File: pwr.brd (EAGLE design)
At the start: 79.5 x 58 mm, 44 parts, among them Q1 IPD65R600C6, T1 750811647, U1 UCC28700, U3 ESP-WROOM-32

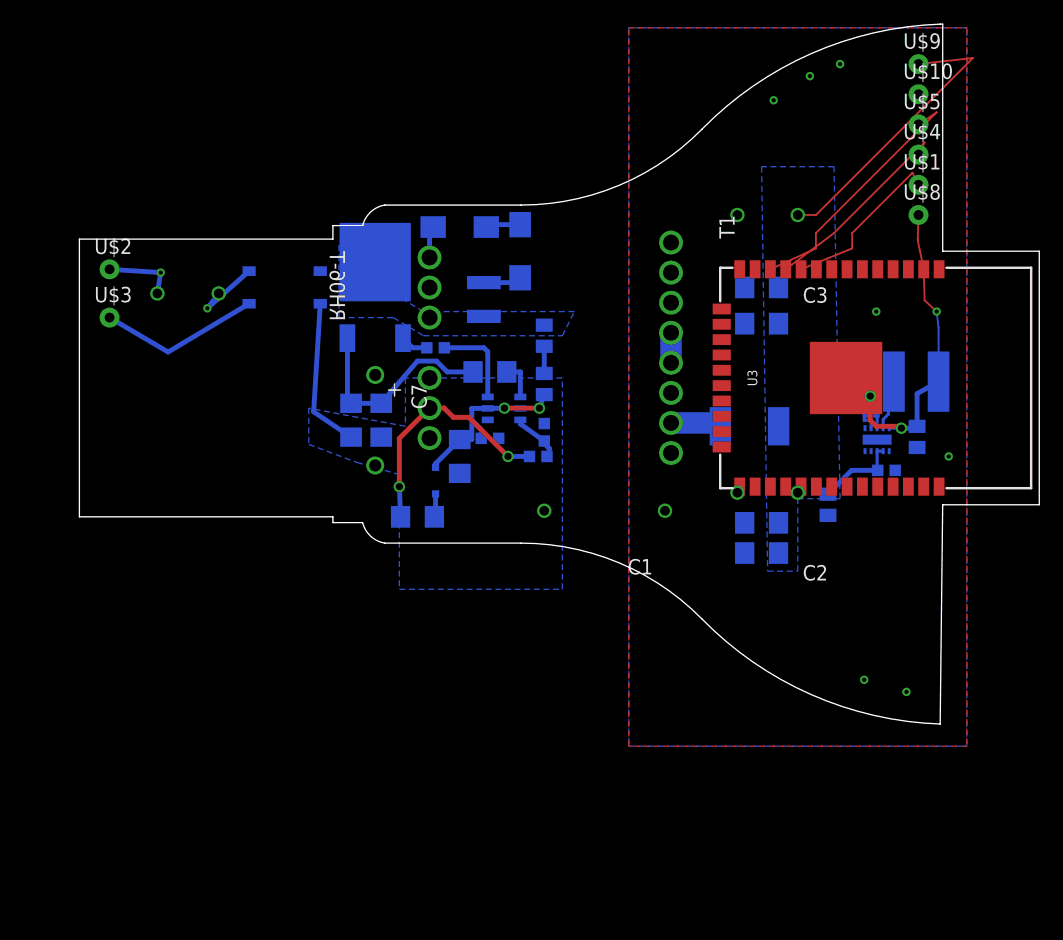
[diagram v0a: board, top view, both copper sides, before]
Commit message: ordered
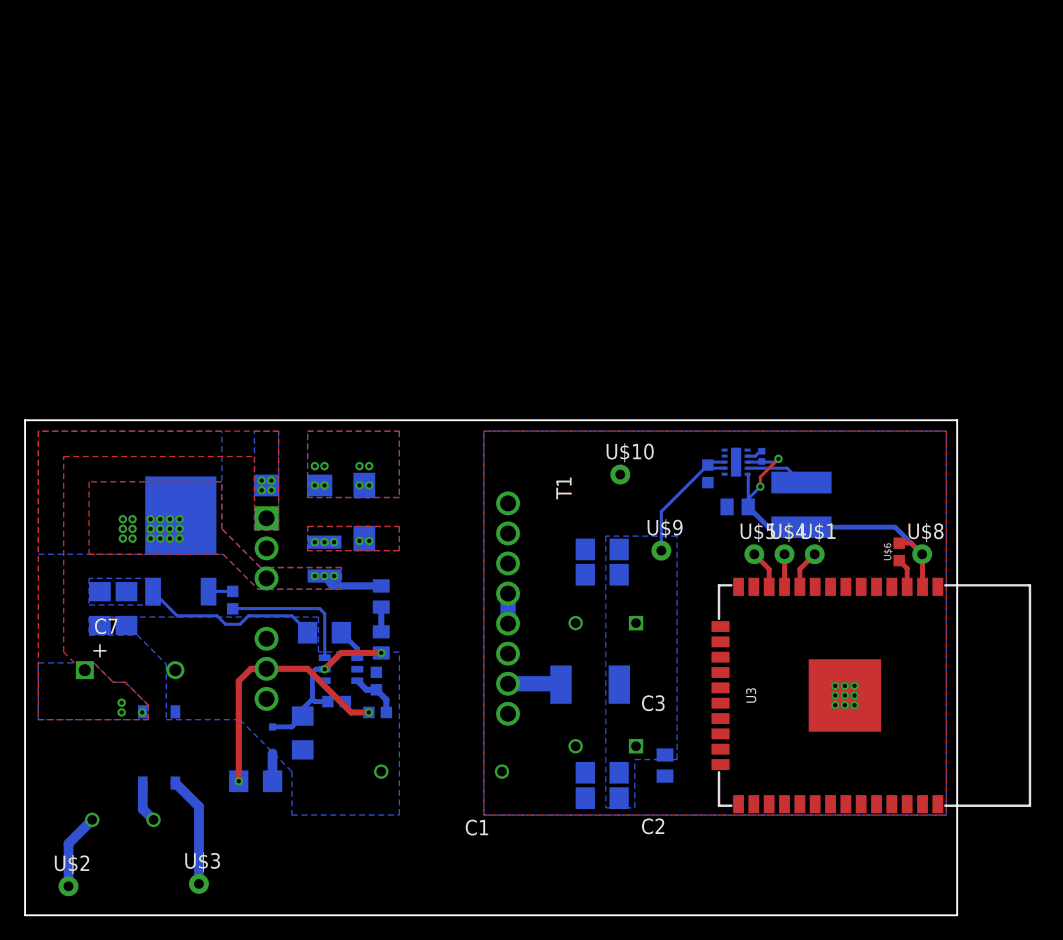
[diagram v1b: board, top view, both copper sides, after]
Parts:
- added U$6: 10k, derek:0603
- moved U$2 51.2 mm to (3.60, 2.40)
- moved U$3 47.5 mm to (14.4, 2.60)
- moved U$9 45.6 mm to (52.7, 30.2)
- moved F1 43.9 mm to (8.10, 7.90)
- moved U$10 40.0 mm to (49.3, 36.5)
- moved D3 39.5 mm to (11.1, 13.9), turned to 180 degrees
- moved U$5 38.1 mm to (60.4, 29.9)
- moved C3 36.4 mm to (48.1, 24.2)
- moved U$4 34.9 mm to (62.9, 29.9)
- moved U$1 31.8 mm to (65.4, 29.9)
- moved C7 29.0 mm to (8.70, 20.3), turned to 0 degrees
- moved U$8 28.1 mm to (74.3, 29.9)
- moved R9 28.0 mm to (6.20, 25.4)
- moved R7 26.8 mm to (17.2, 26.1), turned to 270 degrees
- moved Q1 26.5 mm to (12.9, 31.0)
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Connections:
- new net N$22: U$6.1, U3.3
- net 3.3V: now also U$6.2
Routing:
- net 24V: track 31.5 -> 11.7 mm
- net N$23: track 21.4 -> 3.21 mm
- net N$24: track 16.7 -> 2.70 mm
- net GND: track 12.7 -> 0.00 mm
- net N$21: track 14.0 -> 3.21 mm
- net N$10: track 0.10 -> 5.11 mm, vias 0 -> 21
- net N$2: track 13.4 -> 9.16 mm
- net N$13: track 7.48 -> 11.5 mm
- net N$9: track 3.40 -> 0.00 mm, vias 0 -> 5
- net N$8: track 3.00 -> 0.00 mm, vias 0 -> 8
- net N$3: track 2.82 -> 0.00 mm, vias 0 -> 7
- net N$1: track 6.17 -> 3.42 mm, vias 1 -> 0
- net N$15: track 17.5 -> 14.8 mm
- net N$22: track 0.00 -> 2.45 mm
- net 3.3V: track 29.2 -> 31.5 mm, vias 3 -> 2
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- added copper zone on layer 1, net N$10
- added copper zone on layer 16, net N$15
- added copper zone on layer 1, net N$3
- added copper zone on layer 16, net N$3
- added copper zone on layer 1, net N$8
- added copper zone on layer 16, net N$8
- added copper zone on layer 1, net N$9
- added copper zone on layer 16, net N$9
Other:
- board size 79.5 x 58 mm -> 77.2 x 41 mm
